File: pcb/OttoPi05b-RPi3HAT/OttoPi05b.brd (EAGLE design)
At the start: 56 x 65 mm, 32 parts

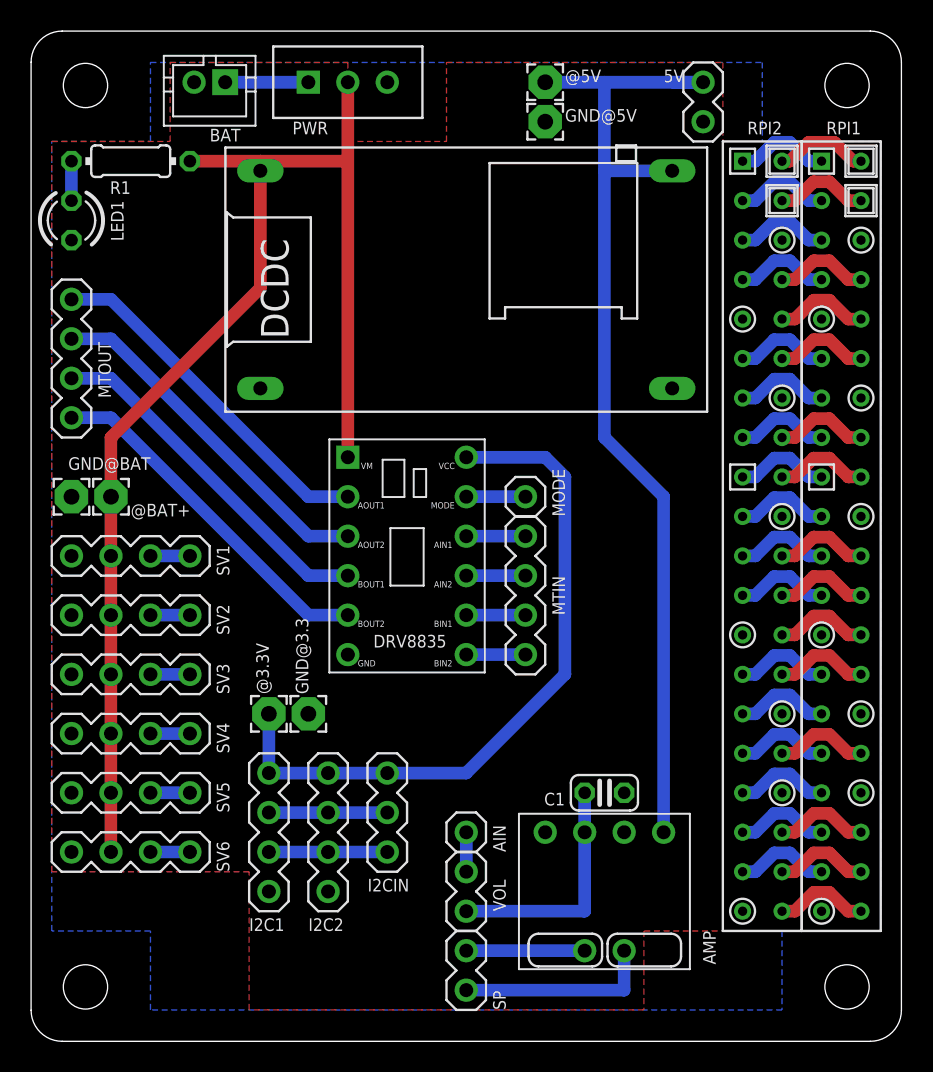
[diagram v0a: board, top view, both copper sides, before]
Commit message: update
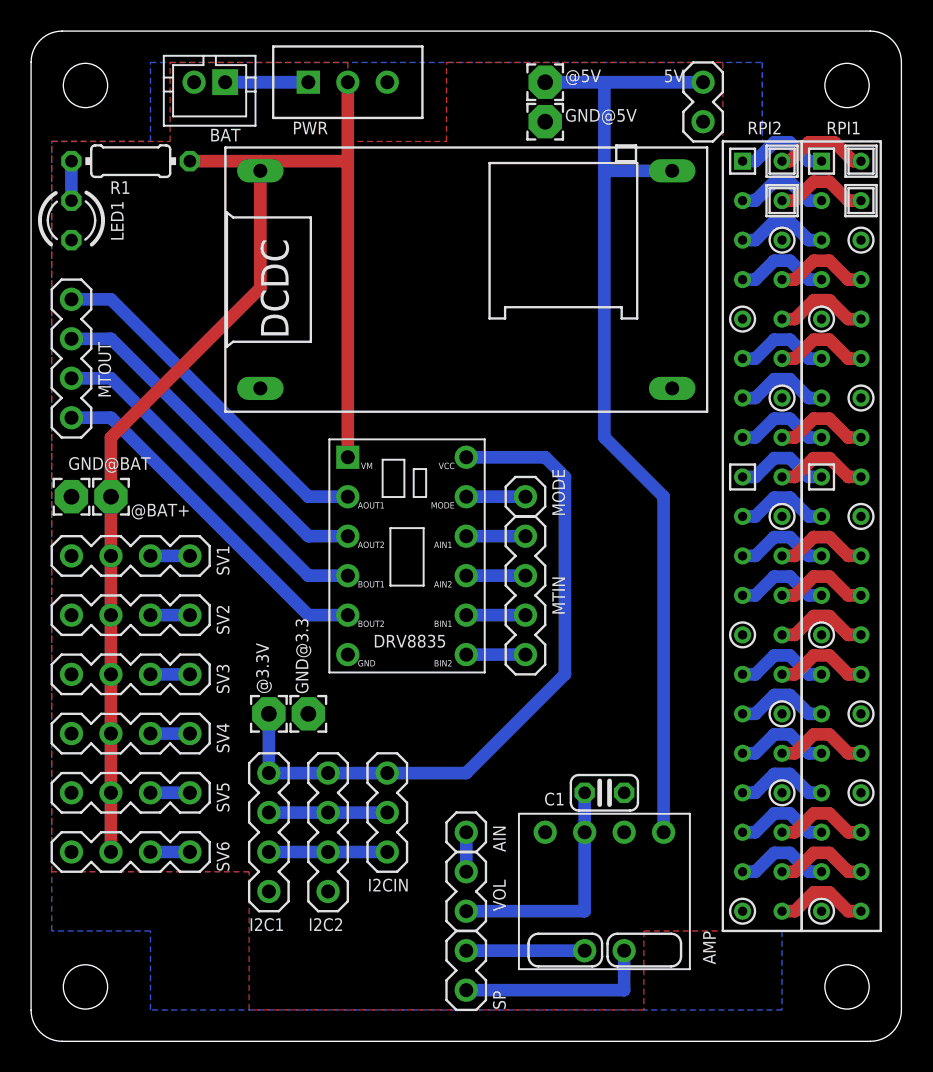
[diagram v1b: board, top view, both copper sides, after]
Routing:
- net +5V: track 66.3 -> 64.4 mm
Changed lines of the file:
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@@
 <contactref element="C1" pad="1"/>
 <contactref element="VOL" pad="2"/>
-<wire x1="0" y1="-24.13" x2="7.62" y2="-24.13" width="0.8128" layer="16"/>
-<wire x1="7.62" y1="-24.13" x2="7.62" y2="-16.51" width="0.8128" layer="16"/>
-<wire x1="7.62" y1="-16.51" x2="7.62" y2="-19.05" width="0" layer="19" extent="1-1"/>
+<wire x1="7.62" y1="-24.13" x2="0" y2="-24.13" width="0.8128" layer="16"/>
+<wire x1="7.62" y1="-16.51" x2="7.62" y2="-19.05" width="0.8128" layer="16"/>
+<wire x1="7.62" y1="-19.05" x2="7.62" y2="-24.13" width="0.8128" layer="16"/>
 </signal>
 <signal name="SP+">
@@
 <wire x1="5.08" y1="29.21" x2="8.89" y2="29.21" width="0.8128" layer="16"/>
 <wire x1="8.89" y1="29.21" x2="15.24" y2="29.21" width="0.8128" layer="16"/>
-<wire x1="15.24" y1="29.21" x2="13.25" y2="29.21" width="0.8128" layer="16"/>
 <contactref element="AMP" pad="V+"/>
 <wire x1="12.7" y1="-19.05" x2="12.7" y2="2.54" width="0.8128" layer="16"/>
